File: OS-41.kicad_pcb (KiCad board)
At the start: 4 copper layers, 65 parts, among them J1 Conn_02x03_Counter_Clockwise, J2 Conn_01x02_Pin, J3 Conn_01x02_Pin, J4 Conn_Coaxial, SW4 SW_Push, U1 BME280, U2 SI4432-B1-FMR, U3 MCP1640x-xCHY, U4 ATGM336H-5N31, U7 STM32F103C8Tx, Y1 32.768KHz 12.5pF, Y2 8MHz 12pF, Y3 30MHz 10pF

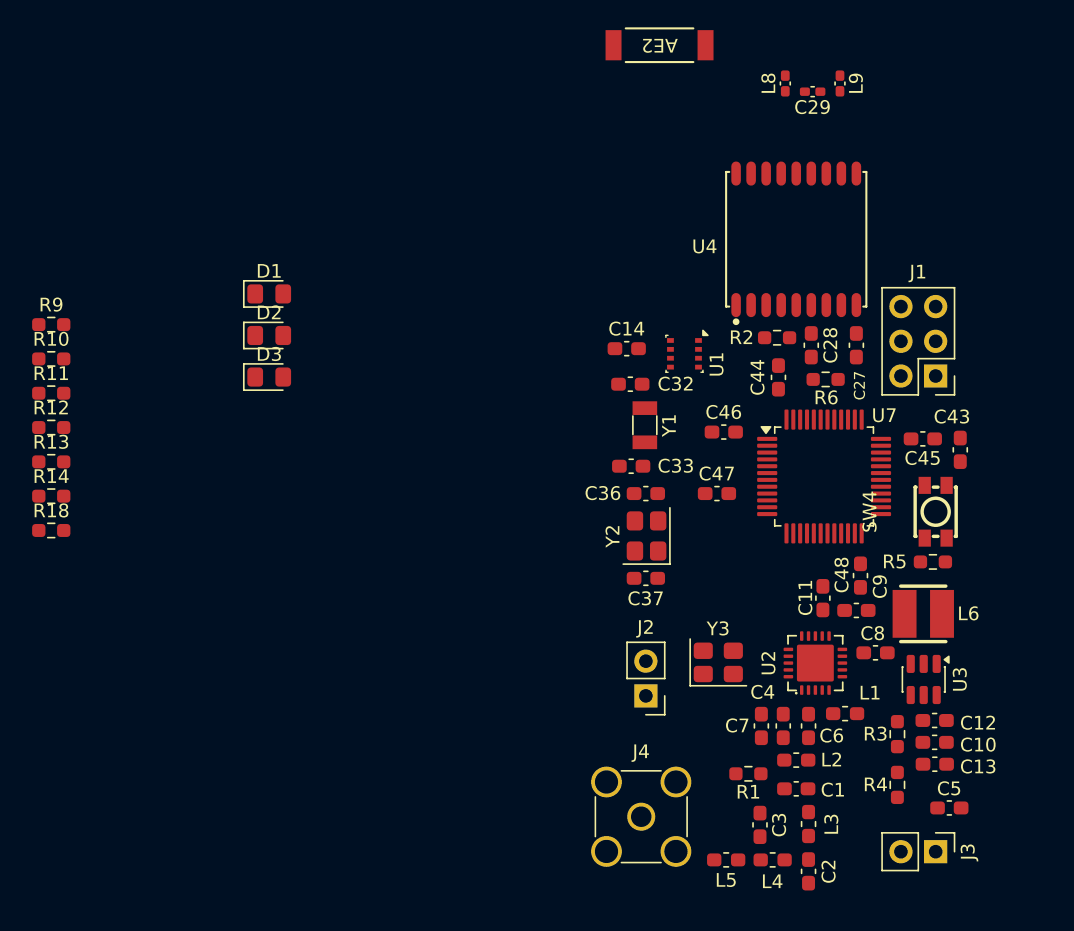
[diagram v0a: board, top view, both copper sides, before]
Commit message: Finished V1 layout!
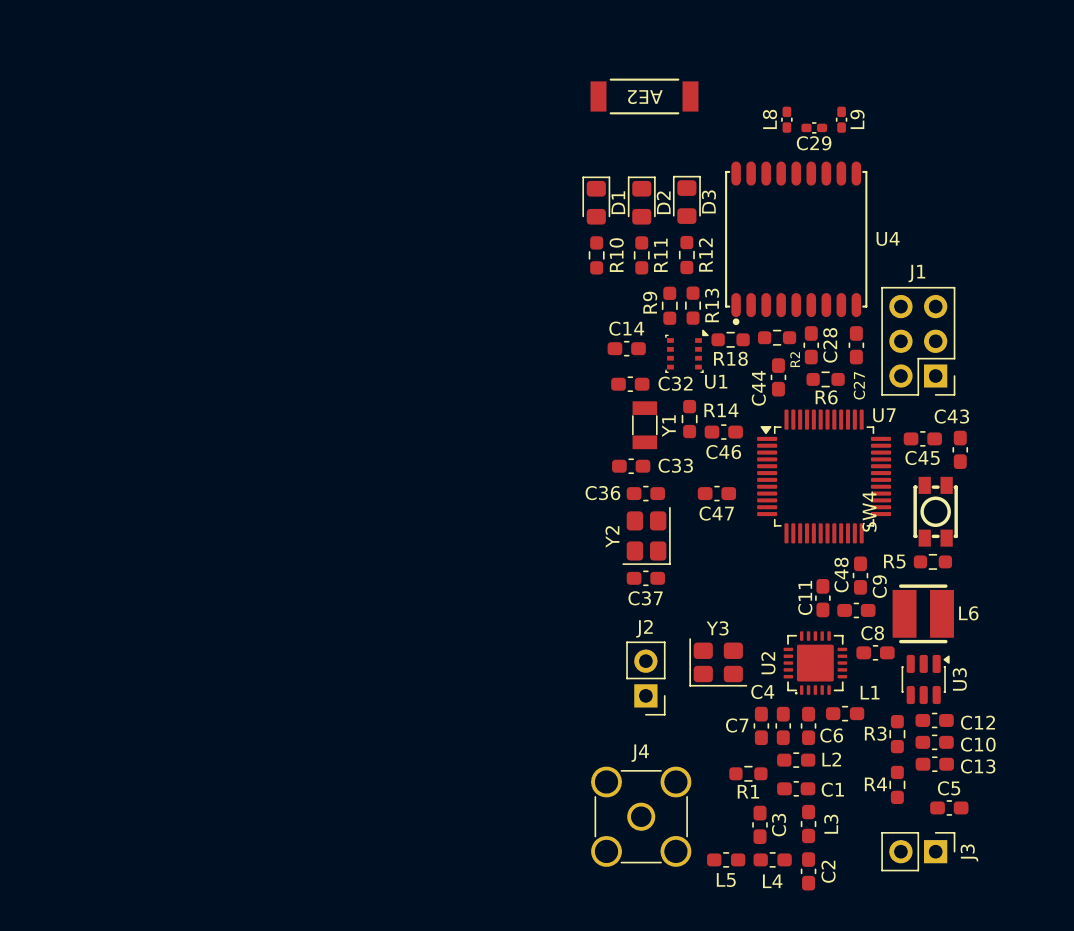
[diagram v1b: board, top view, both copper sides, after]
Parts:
- moved R18 51.6 mm to (139.0, 72.8), turned to 180 degrees
- moved R13 48.3 mm to (136.2, 70.2), turned to -90 degrees
- moved R12 48.2 mm to (135.8, 66.5), turned to -90 degrees
- moved R14 47.0 mm to (136.0, 78.5), turned to -90 degrees
- moved R9 45.3 mm to (134.6, 70.3), turned to 90 degrees
- moved R11 44.4 mm to (132.5, 66.6), turned to -90 degrees
- moved R10 40.6 mm to (129.2, 66.6), turned to 90 degrees
- moved D3 33.1 mm to (135.8, 62.7), turned to -90 degrees
- moved D2 28.9 mm to (132.5, 62.7), turned to -90 degrees
- moved D1 24.8 mm to (129.2, 62.7), turned to -90 degrees
- moved AE2 3.91 mm to (132.7, 55.0)
- moved C29 2.65 mm to (145.1, 57.2)
- moved L8 2.65 mm to (143.1, 56.6)
- moved L9 2.65 mm to (147.1, 56.6)

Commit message: Layout initial done
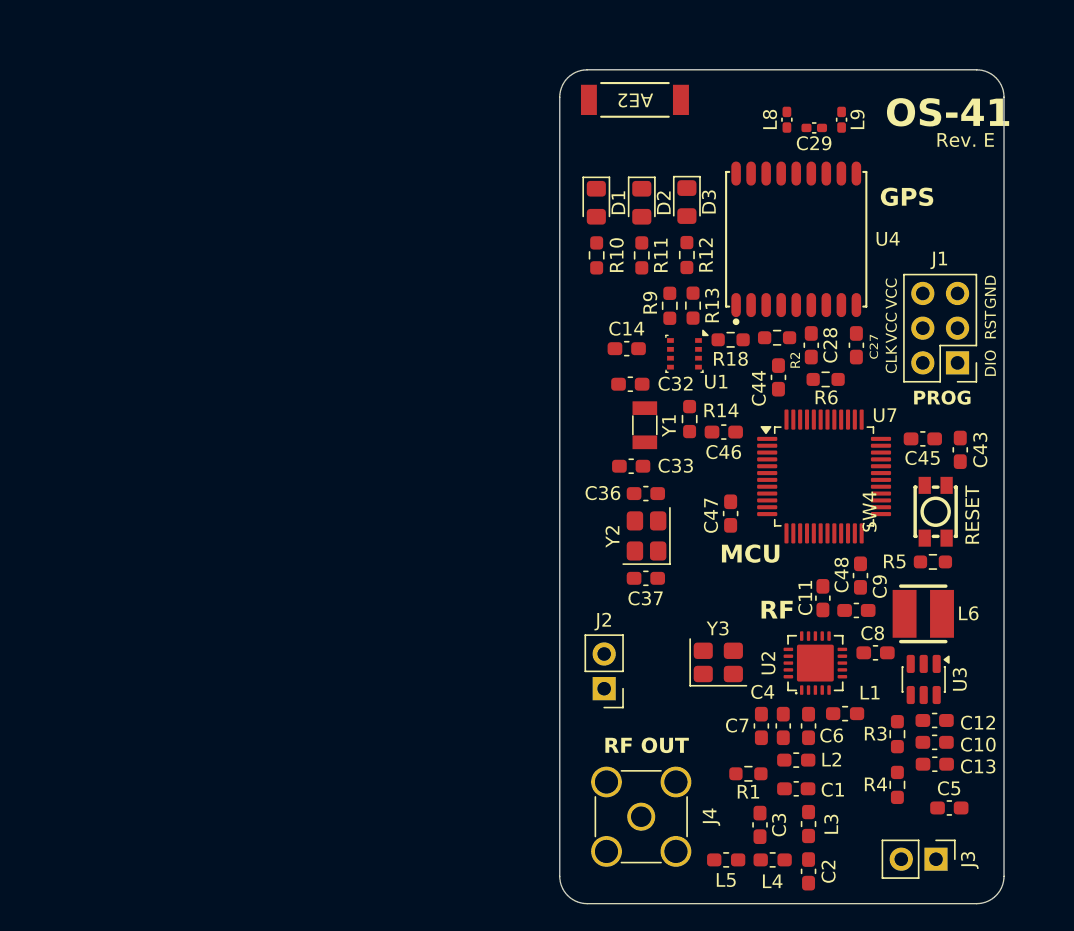
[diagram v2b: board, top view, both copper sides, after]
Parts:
- moved J2 3.09 mm to (129.8, 98.3)
- moved J1 1.87 mm to (155.6, 74.4)
- moved C47 1.77 mm to (139.0, 85.5), turned to 90 degrees
- moved AE2 0.74 mm to (132.0, 55.2)
- moved J3 0.55 mm to (154.0, 110.8)
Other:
- board outline added: 32.5 x 61 mm
- board text added: "CLK"
- board text added: "DIO"
- board text added: "GND"
- board text added: "GPS"
- board text added: "MCU"
- board text added: "OS-41"
- board text added: "PROG"
- board text added: "RESET"
- board text added: "RF"
- board text added: "RF OUT"
- board text added: "RST"
- board text added: "Rev. E"
- board text added: "VCC"
